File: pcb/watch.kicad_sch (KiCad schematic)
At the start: 28 parts, among them J1 USB_C_Receptacle_USB2.0_14P, SW1 SW_Push, SW2 SW_Push, SW3 SW_Push, SW4 SW_Push, U1 nRF52840, U2 USBLC6-2SC6, Y1 32MHz

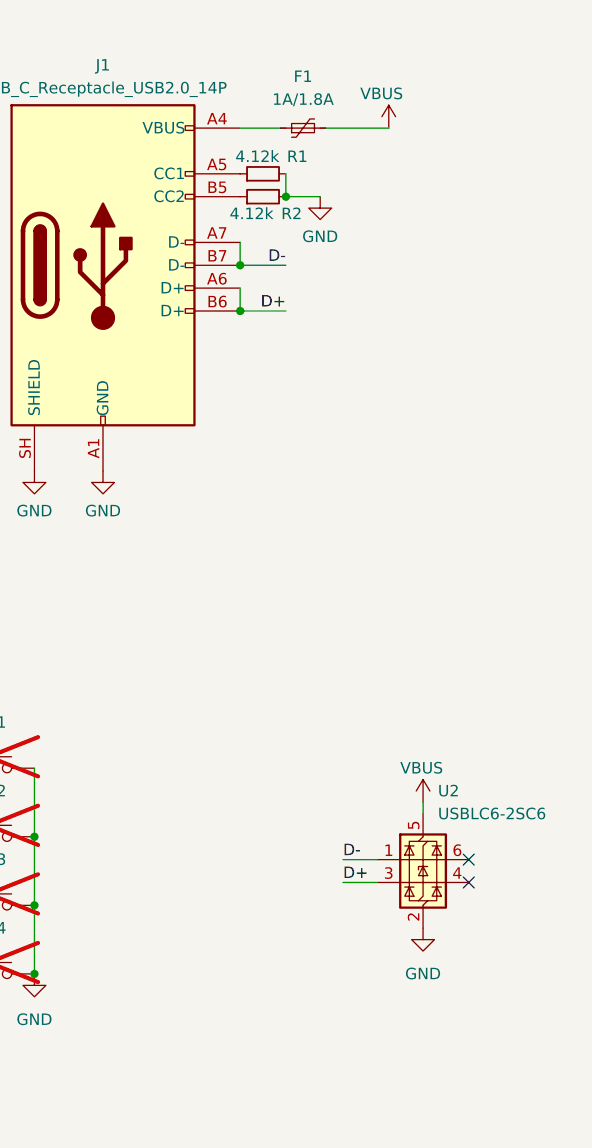
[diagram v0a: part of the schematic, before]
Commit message: starting le leyout
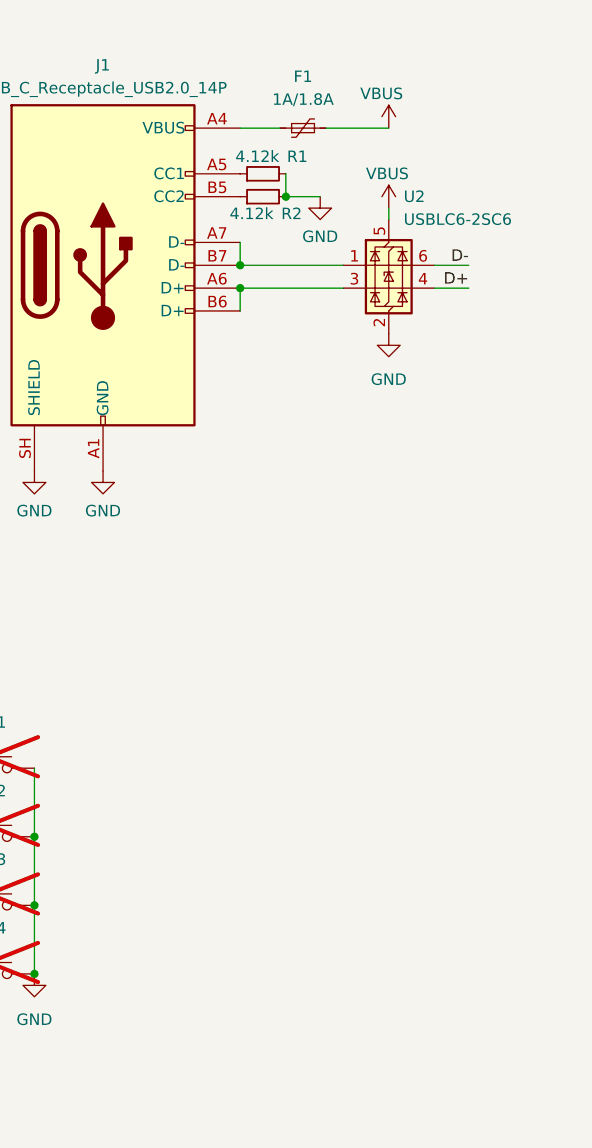
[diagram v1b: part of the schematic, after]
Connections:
- net D+: now also U2.4 (I/O2); no longer J1.A6 (D+), J1.B6 (D+), U2.3 (I/O2)
- net D-: now also U2.6 (I/O1); no longer J1.A7 (D-), J1.B7 (D-), U2.1 (I/O1)
- new net: J1.A7 (D-), J1.B7 (D-), U2.1 (I/O1)
- new net: J1.A6 (D+), J1.B6 (D+), U2.3 (I/O2)
- no-connect marks 16 -> 14
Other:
- moved on the sheet: U2
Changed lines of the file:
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@@
 	)
 	(junction
-		(at 226.06 63.5)
+		(at 226.06 60.96)
 		(diameter 0)
 		(color 0 0 0 0)
 	)
 	(junction
-		(at 226.06 58.42)
+		(at 66.04 124.46)
 		(diameter 0)
 		(color 0 0 0 0)
 	)
 	(junction
-		(at 66.04 124.46)
+		(at 226.06 58.42)
 		(diameter 0)
 		(color 0 0 0 0)
@@
 	)
 	(no_connect
-		(at 251.46 127)
-	)
-	(no_connect
 		(at 139.7 81.28)
 	)
@@
 	)
 	(no_connect
-		(at 251.46 124.46)
-	)
-	(no_connect
 		(at 88.9 48.26)
 	)
@@
 	(wire
 		(pts
-			(xy 237.49 127) (xy 241.3 127)
+			(xy 113.665 20.32) (xy 113.665 22.225)
 		)
 		(stroke
@@
 	(wire
 		(pts
-			(xy 113.665 20.32) (xy 113.665 22.225)
+			(xy 53.34 114.3) (xy 55.88 114.3)
 		)
 		(stroke
@@
 	(wire
 		(pts
-			(xy 53.34 114.3) (xy 55.88 114.3)
+			(xy 139.7 180.34) (xy 143.51 180.34)
 		)
 		(stroke
@@
 	(wire
 		(pts
-			(xy 139.7 180.34) (xy 143.51 180.34)
+			(xy 146.685 41.91) (xy 153.67 41.91)
 		)
 		(stroke
@@
 	(wire
 		(pts
-			(xy 146.685 41.91) (xy 153.67 41.91)
+			(xy 73.66 46.355) (xy 86.36 46.355)
 		)
 		(stroke
@@
 	(wire
 		(pts
-			(xy 73.66 46.355) (xy 86.36 46.355)
+			(xy 53.34 119.38) (xy 60.96 119.38)
 		)
 		(stroke
@@
 	(wire
 		(pts
-			(xy 53.34 119.38) (xy 60.96 119.38)
+			(xy 226.06 60.96) (xy 237.49 60.96)
 		)
 		(stroke
@@
 	(wire
 		(pts
-			(xy 86.36 46.355) (xy 86.36 48.26)
+			(xy 247.65 60.96) (xy 251.46 60.96)
 		)
 		(stroke
@@
 	(wire
 		(pts
-			(xy 74.93 20.32) (xy 74.93 22.225)
+			(xy 86.36 46.355) (xy 86.36 48.26)
 		)
 		(stroke
@@
 	(wire
 		(pts
-			(xy 226.06 60.96) (xy 226.06 63.5)
+			(xy 74.93 20.32) (xy 74.93 22.225)
 		)
 		(stroke
@@
 	(wire
 		(pts
-			(xy 106.68 20.32) (xy 106.68 48.26)
+			(xy 226.06 60.96) (xy 226.06 63.5)
 		)
 		(stroke
@@
 	(wire
 		(pts
-			(xy 97.155 20.32) (xy 97.155 22.225)
+			(xy 106.68 20.32) (xy 106.68 48.26)
 		)
 		(stroke
@@
 	(wire
 		(pts
-			(xy 226.06 63.5) (xy 231.14 63.5)
+			(xy 97.155 20.32) (xy 97.155 22.225)
 		)
 		(stroke
@@
 	(wire
 		(pts
+			(xy 247.65 58.42) (xy 251.46 58.42)
+		)
+		(stroke
+			(width 0)
+			(type default)
+		)
+	)
+	(wire
+		(pts
 			(xy 235.585 43.18) (xy 242.57 43.18)
 		)
@@
 	(wire
 		(pts
-			(xy 226.06 58.42) (xy 231.14 58.42)
-		)
-		(stroke
-			(width 0)
-			(type default)
-		)
-	)
-	(wire
-		(pts
 			(xy 124.46 45.72) (xy 133.985 45.72)
 		)
@@
 	(wire
 		(pts
-			(xy 246.38 118.11) (xy 246.38 119.38)
+			(xy 242.57 52.07) (xy 242.57 53.34)
 		)
 		(stroke
@@
 	(wire
 		(pts
-			(xy 111.76 48.26) (xy 111.76 35.56)
+			(xy 237.49 58.42) (xy 226.06 58.42)
 		)
 		(stroke
@@
 	(wire
 		(pts
-			(xy 91.44 43.18) (xy 91.44 48.26)
+			(xy 111.76 48.26) (xy 111.76 35.56)
 		)
 		(stroke
@@
 	(wire
 		(pts
-			(xy 62.865 46.99) (xy 62.865 43.18)
+			(xy 91.44 43.18) (xy 91.44 48.26)
 		)
 		(stroke
@@
 	(wire
 		(pts
-			(xy 237.49 124.46) (xy 241.3 124.46)
+			(xy 62.865 46.99) (xy 62.865 43.18)
 		)
 		(stroke
@@
 		)
 	)
-	(label "D-"
-		(at 237.49 124.46 0)
-		(effects
-			(font
-				(size 1.27 1.27)
-			)
-			(justify left bottom)
-		)
-	)
 	(label "VDD_nRF"
 		(at 52.07 20.32 0)
@@
 		)
 	)
-	(label "D-"
-		(at 231.14 58.42 180)
+	(label "DEC4"
+		(at 153.67 41.91 180)
 		(effects
 			(font
@@
 		)
 	)
-	(label "D+"
-		(at 231.14 63.5 180)
+	(label "VDD_nRF"
+		(at 133.985 45.72 180)
 		(effects
 			(font
@@
 		)
 	)
-	(label "DEC4"
-		(at 153.67 41.91 180)
+	(label "D-"
+		(at 251.46 58.42 180)
 		(effects
 			(font
@@
 		)
 	)
-	(label "VDD_nRF"
-		(at 133.985 45.72 180)
+	(label "D+"
+		(at 251.46 60.96 180)
 		(effects
 			(font
@@
 	)
 	(label "D+"
-		(at 237.49 127 0)
-		(effects
-			(font
-				(size 1.27 1.27)
-			)
-			(justify left bottom)
-		)
-	)
-	(label "D+"
 		(at 143.51 182.88 180)
 		(effects
@@
 	(symbol
 		(lib_id "power:GND")
-		(at 246.38 132.08 0)
+		(at 242.57 66.04 0)
 		(unit 1)
 		(body_style 1)
@@
 		(dnp no)
 		(property "Reference" "#PWR022"
-			(at 246.38 138.43 0)
+			(at 242.57 72.39 0)
 			(hide yes)
 			(show_name no)
@@
 		)
 		(property "Value" "GND"
-			(at 246.38 137.16 0)
+			(at 242.57 71.12 0)
 			(show_name no)
 			(do_not_autoplace no)
@@
 		)
 		(property "Footprint" ""
-			(at 246.38 132.08 0)
+			(at 242.57 66.04 0)
 			(hide yes)
 			(show_name no)
@@
 		)
 		(property "Datasheet" ""
-			(at 246.38 132.08 0)
+			(at 242.57 66.04 0)
 			(hide yes)
 			(show_name no)
@@
 		)
 		(property "Description" "Power symbol creates a global label with name \"GND\" , ground"
-			(at 246.38 132.08 0)
+			(at 242.57 66.04 0)
 			(hide yes)
 			(show_name no)
@@
 	(symbol
 		(lib_id "Power_Protection:USBLC6-2SC6")
-		(at 246.38 124.46 0)
+		(at 242.57 58.42 0)
 		(unit 1)
 		(body_style 1)
@@
 		(fields_autoplaced yes)
 		(property "Reference" "U2"
-			(at 248.0311 116.84 0)
+			(at 244.2211 50.8 0)
 			(show_name no)
 			(do_not_autoplace no)
@@
 		)
 		(property "Value" "USBLC6-2SC6"
-			(at 248.0311 119.38 0)
+			(at 244.2211 53.34 0)
 			(show_name no)
 			(do_not_autoplace no)
@@
 		)
 		(property "Footprint" "Package_TO_SOT_SMD:SOT-23-6"
-			(at 247.65 130.81 0)
+			(at 243.84 64.77 0)
 			(hide yes)
 			(show_name no)
@@
 		)
 		(property "Datasheet" "https://www.st.com/resource/en/datasheet/usblc6-2.pdf"
-			(at 247.65 132.715 0)
+			(at 243.84 66.675 0)
 			(hide yes)
 			(show_name no)
@@
 		)
 		(property "Description" "Very low capacitance ESD protection diode, 2 data-line, SOT-23-6"
-			(at 246.38 124.46 0)
+			(at 242.57 58.42 0)
 			(hide yes)
 			(show_name no)
@@
 		)
 		(property "KLC_S3.3" ""
-			(at 246.38 124.46 0)
+			(at 242.57 58.42 0)
 			(hide yes)
 			(show_name no)
@@
 		)
 		(property "KLC_S4.1" ""
-			(at 246.38 124.46 0)
+			(at 242.57 58.42 0)
 			(hide yes)
 			(show_name no)
@@
 		)
 		(property "LCSC Part" "C7519"
-			(at 246.38 124.46 0)
+			(at 242.57 58.42 0)
 			(hide yes)
 			(show_name no)
@@
 		)
 		(property "LCSC" ""
-			(at 246.38 124.46 0)
+			(at 242.57 58.42 0)
 			(hide yes)
 			(show_name no)
@@
 		)
 		(property "Manufacturer Part" ""
-			(at 246.38 124.46 0)
+			(at 242.57 58.42 0)
 			(hide yes)
 			(show_name no)
@@
 	(symbol
 		(lib_id "power:+5V")
-		(at 246.38 118.11 0)
+		(at 242.57 52.07 0)
 		(unit 1)
 		(body_style 1)
@@
 		(dnp no)
 		(property "Reference" "#PWR021"
-			(at 246.38 121.92 0)
+			(at 242.57 55.88 0)
 			(hide yes)
 			(show_name no)
@@
 		)
 		(property "Value" "VBUS"
-			(at 243.84 114.3 0)
+			(at 240.03 48.26 0)
 			(show_name no)
 			(do_not_autoplace no)
@@
 		)
 		(property "Footprint" ""
-			(at 246.38 118.11 0)
+			(at 242.57 52.07 0)
 			(hide yes)
 			(show_name no)
@@
 		)
 		(property "Datasheet" ""
-			(at 246.38 118.11 0)
+			(at 242.57 52.07 0)
 			(hide yes)
 			(show_name no)
@@
 		)
 		(property "Description" "Power symbol creates a global label with name \"+5V\""
-			(at 246.38 118.11 0)
+			(at 242.57 52.07 0)
 			(hide yes)
 			(show_name no)

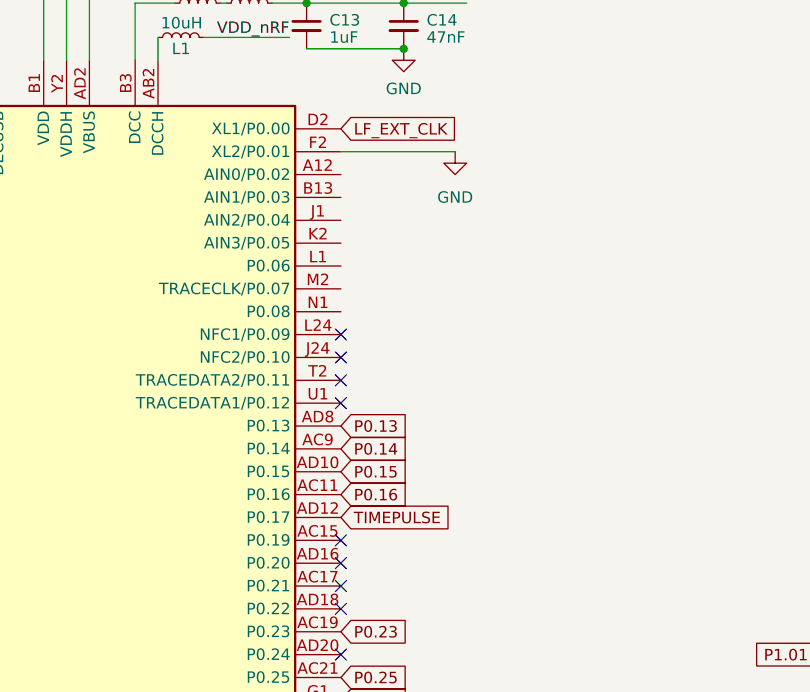
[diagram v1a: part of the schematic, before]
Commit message: mogus
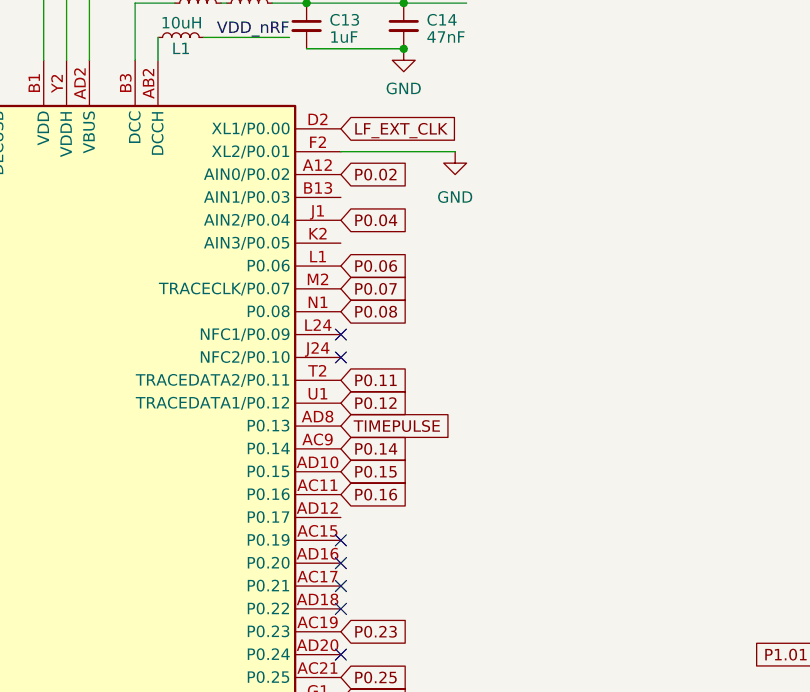
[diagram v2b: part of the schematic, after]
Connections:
- net P0.13 is gone; now on net TIMEPULSE: U1.AD8 (P0.13)
- net TIMEPULSE: no longer U1.AD12 (P0.17)
- net P0.02: now reaches U1.A12 (AIN0/P0.02)
- net P0.04: now reaches U1.J1 (AIN2/P0.04)
- net P0.06: now reaches U1.L1 (P0.06)
- net P0.07: now reaches U1.M2 (TRACECLK/P0.07)
- net P0.08: now reaches U1.N1 (P0.08)
- net P0.11: now reaches U1.T2 (TRACEDATA2/P0.11)
- net P0.12: now reaches U1.U1 (TRACEDATA1/P0.12)
- no-connect marks 14 -> 12
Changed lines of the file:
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@@
 	)
 	(no_connect
-		(at 139.7 86.36)
-	)
-	(no_connect
-		(at 139.7 83.82)
-	)
-	(no_connect
 		(at 73.66 73.66)
 	)
@@
 		)
 	)
+	(global_label "P0.12"
+		(shape input)
+		(at 139.7 86.36 0)
+		(fields_autoplaced yes)
+		(effects
+			(font
+				(size 1.27 1.27)
+			)
+			(justify left)
+		)
+		(property "Intersheetrefs" "${INTERSHEET_REFS}"
+			(at 148.1885 86.36 0)
+			(hide yes)
+			(show_name no)
+			(do_not_autoplace no)
+			(effects
+				(font
+					(size 1.27 1.27)
+				)
+				(justify left)
+			)
+		)
+	)
 	(global_label "P0.16"
 		(shape input)
@@
 		)
 	)
-	(global_label "P0.13"
+	(global_label "P1.11"
 		(shape input)
-		(at 139.7 88.9 0)
+		(at 139.7 165.1 0)
 		(fields_autoplaced yes)
 		(effects
@@
 		)
 		(property "Intersheetrefs" "${INTERSHEET_REFS}"
-			(at 148.1885 88.9 0)
+			(at 148.1885 165.1 0)
 			(hide yes)
 			(show_name no)
@@
 		)
 	)
-	(global_label "P1.11"
+	(global_label "P1.01"
 		(shape input)
-		(at 139.7 165.1 0)
+		(at 139.7 139.7 0)
 		(fields_autoplaced yes)
 		(effects
@@
 		)
 		(property "Intersheetrefs" "${INTERSHEET_REFS}"
-			(at 148.1885 165.1 0)
+			(at 148.1885 139.7 0)
 			(hide yes)
 			(show_name no)
@@
 		)
 	)
-	(global_label "P1.01"
+	(global_label "P0.02"
 		(shape input)
-		(at 139.7 139.7 0)
+		(at 139.7 60.96 0)
 		(fields_autoplaced yes)
 		(effects
@@
 		)
 		(property "Intersheetrefs" "${INTERSHEET_REFS}"
-			(at 148.1885 139.7 0)
+			(at 148.1885 60.96 0)
+			(hide yes)
+			(show_name no)
+			(do_not_autoplace no)
+			(effects
+				(font
+					(size 1.27 1.27)
+				)
+				(justify left)
+			)
+		)
+	)
+	(global_label "P0.04"
+		(shape input)
+		(at 139.7 66.04 0)
+		(fields_autoplaced yes)
+		(effects
+			(font
+				(size 1.27 1.27)
+			)
+			(justify left)
+		)
+		(property "Intersheetrefs" "${INTERSHEET_REFS}"
+			(at 148.1885 66.04 0)
 			(hide yes)
 			(show_name no)
@@
 		)
 	)
+	(global_label "P0.11"
+		(shape input)
+		(at 139.7 83.82 0)
+		(fields_autoplaced yes)
+		(effects
+			(font
+				(size 1.27 1.27)
+			)
+			(justify left)
+		)
+		(property "Intersheetrefs" "${INTERSHEET_REFS}"
+			(at 148.1885 83.82 0)
+			(hide yes)
+			(show_name no)
+			(do_not_autoplace no)
+			(effects
+				(font
+					(size 1.27 1.27)
+				)
+				(justify left)
+			)
+		)
+	)
 	(global_label "LF_EXT_CLK"
 		(shape input)
@@
 		)
 	)
+	(global_label "TIMEPULSE"
+		(shape input)
+		(at 139.7 88.9 0)
+		(fields_autoplaced yes)
+		(effects
+			(font
+				(size 1.27 1.27)
+			)
+			(justify left)
+		)
+		(property "Intersheetrefs" "${INTERSHEET_REFS}"
+			(at 152.8451 88.9 0)
+			(hide yes)
+			(show_name no)
+			(do_not_autoplace no)
+			(effects
+				(font
+					(size 1.27 1.27)
+				)
+				(justify left)
+			)
+		)
+	)
 	(global_label "P0.14"
 		(shape input)
@@
 		)
 	)
+	(global_label "P0.06"
+		(shape input)
+		(at 139.7 71.12 0)
+		(fields_autoplaced yes)
+		(effects
+			(font
+				(size 1.27 1.27)
+			)
+			(justify left)
+		)
+		(property "Intersheetrefs" "${INTERSHEET_REFS}"
+			(at 148.1885 71.12 0)
+			(hide yes)
+			(show_name no)
+			(do_not_autoplace no)
+			(effects
+				(font
+					(size 1.27 1.27)
+				)
+				(justify left)
+			)
+		)
+	)
 	(global_label "P1.12"
 		(shape input)
@@
 		)
 	)
-	(global_label "TIMEPULSE"
+	(global_label "P0.08"
 		(shape input)
-		(at 139.7 99.06 0)
+		(at 139.7 76.2 0)
 		(fields_autoplaced yes)
 		(effects
@@
 		)
 		(property "Intersheetrefs" "${INTERSHEET_REFS}"
-			(at 152.8451 99.06 0)
+			(at 148.1885 76.2 0)
 			(hide yes)
 			(show_name no)
@@
 			(hide yes)
 			(show_name no)
+			(do_not_autoplace no)
+			(effects
+				(font
+					(size 1.27 1.27)
+				)
+				(justify left)
+			)
+		)
+	)
+	(global_label "P0.07"
+		(shape input)
+		(at 139.7 73.66 0)
+		(fields_autoplaced yes)
+		(effects
+			(font
+				(size 1.27 1.27)
+			)
+			(justify left)
+		)
+		(property "Intersheetrefs" "${INTERSHEET_REFS}"
+			(at 148.1885 73.66 0)
+			(hide yes)
+			(show_name no)
